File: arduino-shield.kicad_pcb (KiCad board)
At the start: 2 copper layers, 429 parts

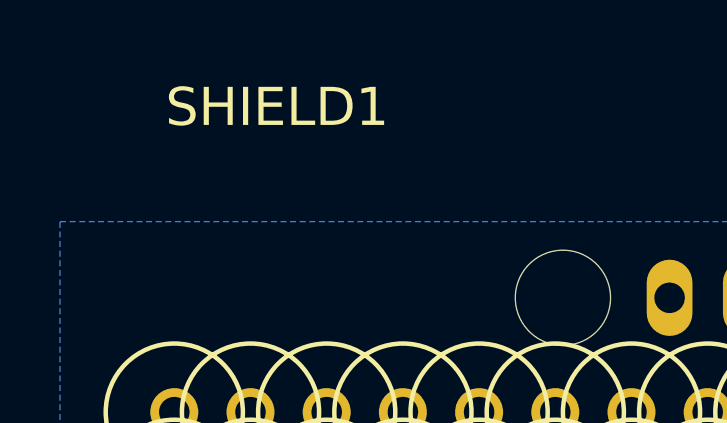
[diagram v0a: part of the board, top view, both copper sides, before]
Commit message: KiCad 6.0.3 format.
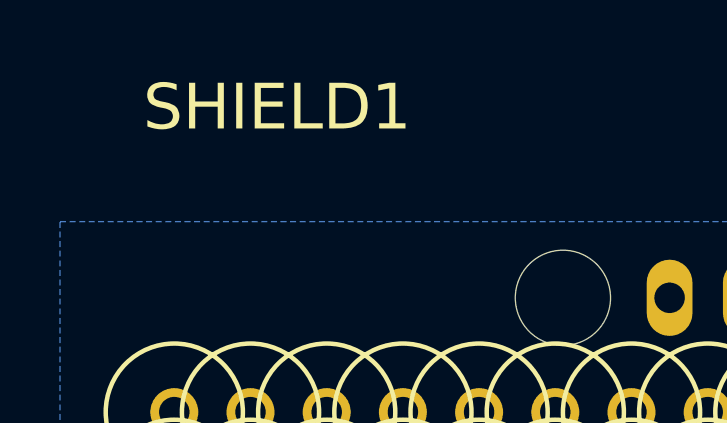
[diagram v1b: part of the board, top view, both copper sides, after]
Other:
- net class Default removed
